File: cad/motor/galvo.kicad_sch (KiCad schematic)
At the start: 14 parts, among them Q13 NMOS, U1 ${SIM.PARAMS}, U2 ${SIM.PARAMS}

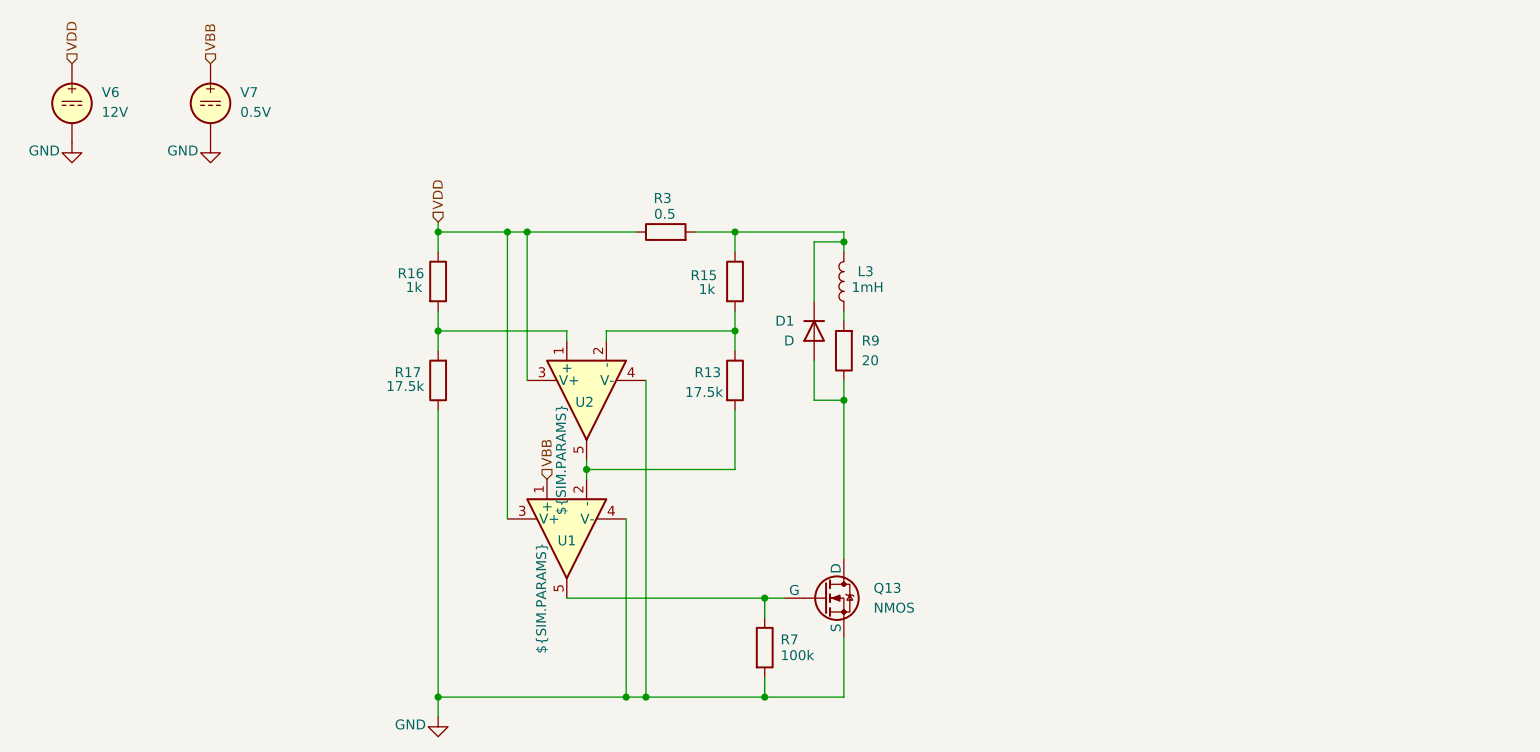
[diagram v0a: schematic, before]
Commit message: schema
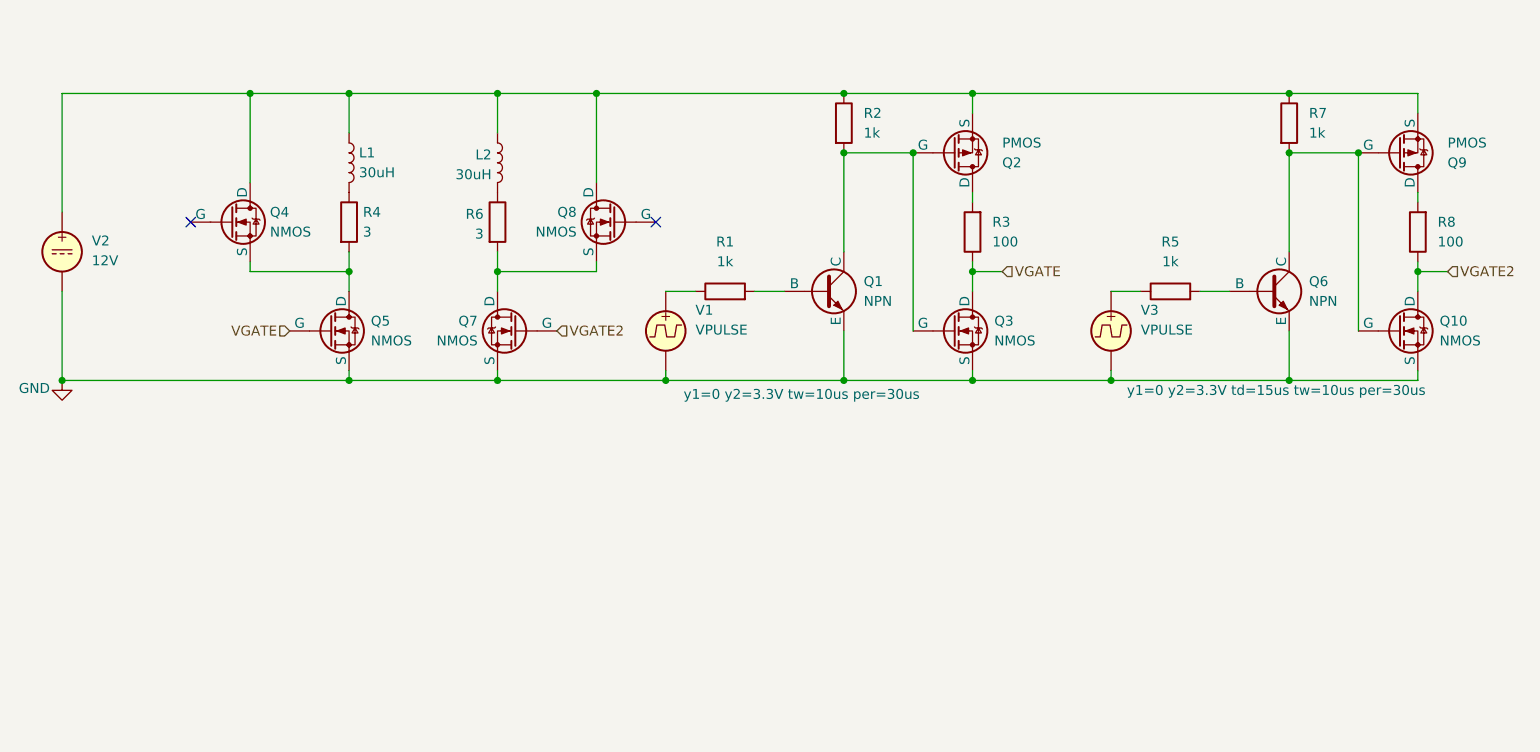
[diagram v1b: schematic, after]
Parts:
- removed D1: D, symbol Device:D
- removed L3: 1mH, symbol Device:L
- removed Q13: NMOS, symbol Simulation_SPICE:NMOS
- removed R13, R17: 17.5k, symbol Device:R
- removed R15, R16: 1k, symbol Device:R
- removed R9: 20, symbol Device:R
- removed U1, U2: ${SIM.PARAMS}, symbol Simulation_SPICE:OPAMP
- removed V6: 12V, symbol Simulation_SPICE:VDC
- removed V7: 0.5V, symbol Simulation_SPICE:VDC
- added L1, L2: 30uH, symbol Device:L
- added Q1, Q6: NPN, symbol Simulation_SPICE:NPN
- added Q10, Q3, Q4, Q5, Q7, Q8: NMOS, symbol Simulation_SPICE:NMOS
- added Q2, Q9: PMOS, symbol Simulation_SPICE:PMOS
- added R1, R2, R5: 1k, symbol Device:R
- added R4, R6: 3, symbol Device:R
- added R8: 100, symbol Device:R
- added V1, V3: VPULSE, symbol Simulation_SPICE:VPULSE
- added V2: 12V, symbol Simulation_SPICE:VDC
- R3: value 0.5 -> 100
- R7: value 100k -> 1k
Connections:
- net GND: now also Q1.3 (E), Q10.3 (S), Q3.3 (S), Q5.3 (S), Q6.3 (E), Q7.3 (S), V1.2, V2.2, V3.2; no longer R7.2
- net at R3.2: now also Q2.1 (D)
- net at R7.1: now also L1.1, L2.1, Q2.3 (S), Q4.1 (D), Q8.1 (D), Q9.3 (S), R2.1, V2.1
- net VDD renamed VGATE
- net VGATE: now also Q3.1 (D), Q5.2 (G)
- new net: R1.1, V1.1
- new net: L2.2, R6.1
- new net: Q7.1 (D), Q8.3 (S), R6.2
- new net: Q1.1 (C), Q2.2 (G), Q3.2 (G), R2.2
- new net: Q9.1 (D), R8.2
- new net: Q10.2 (G), Q6.1 (C), Q9.2 (G), R7.2
- new net: Q6.2 (B), R5.2
- new net: R5.1, V3.1
- new net: Q4.3 (S), Q5.1 (D), R4.2
- new net: L1.2, R4.1
- new net: Q1.2 (B), R1.2
- new net VGATE2: Q10.1 (D), Q7.2 (G), R8.1
- no-connect marks 0 -> 2
